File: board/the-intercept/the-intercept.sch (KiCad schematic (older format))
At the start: 35 parts, among them J1 USB_B_Micro, Q1 Q_Photo_NPN, SW1 SW_Push, SW2 SW_Push, U1 ESP32-WROOM-32D, U2 93LCxxB, U3 FT232H, U4 LM1117-3.3, Y1 12MHz

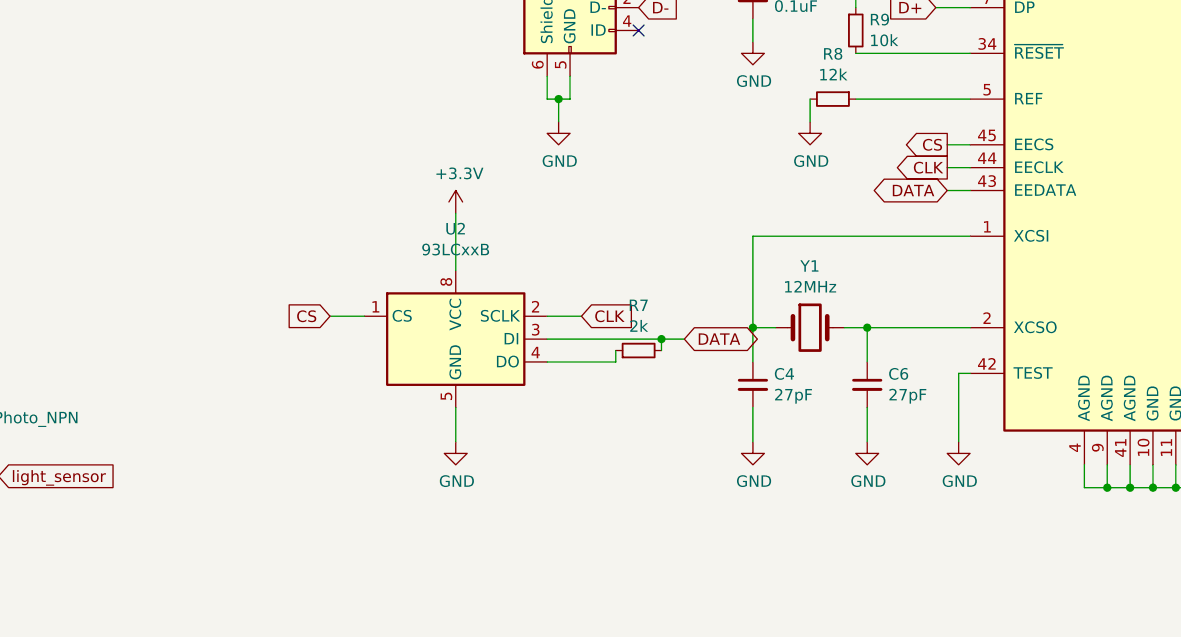
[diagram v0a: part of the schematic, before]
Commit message: Revision two of the board
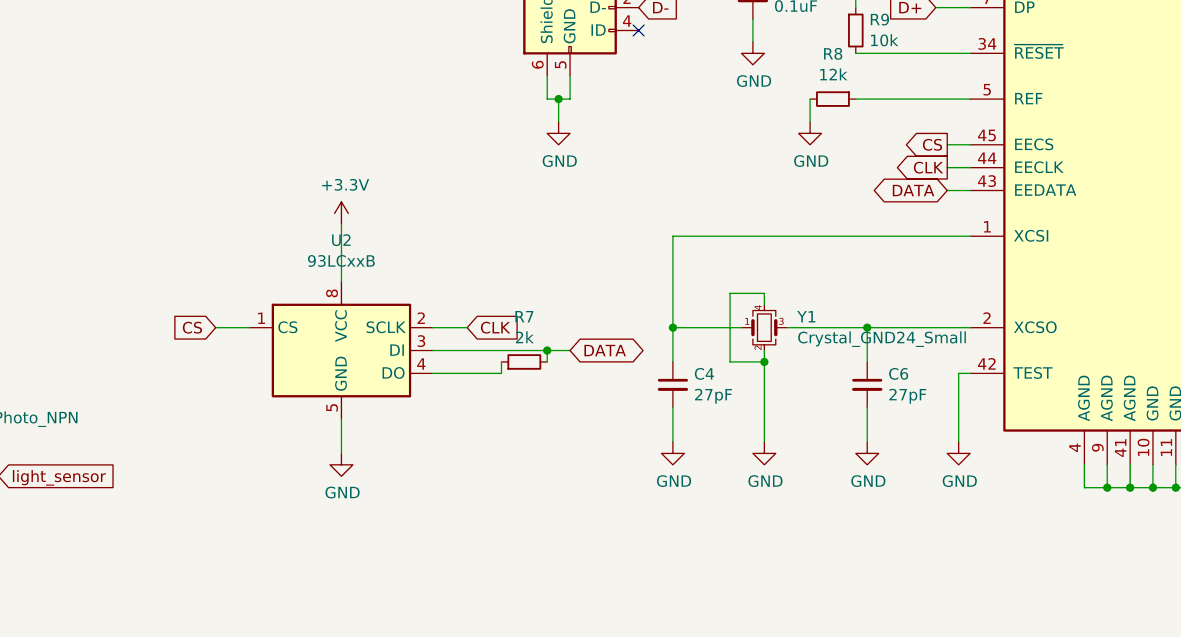
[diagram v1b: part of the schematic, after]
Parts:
- removed Y1: 12MHz, Crystal:Crystal_SMD_Abracon_ABM8G-4Pin_3.2x2.5mm, symbol Device:Crystal
- added Y1: Crystal_GND24_Small, Crystal:Crystal_SMD_Abracon_ABM8G-4Pin_3.2x2.5mm, symbol Device:Crystal_GND24_Small
- U2: footprint Package_SO:SOIC-8-1EP_3.9x4.9mm_P1.27mm_EP2.29x3mm -> Package_SO:SOIC-8_3.9x4.9mm_P1.27mm
- U3: footprint Package_QFP:LQFP-48-1EP_7x7mm_P0.5mm_EP3.6x3.6mm -> Package_QFP:LQFP-48_7x7mm_P0.5mm
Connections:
- net GND: now also Y1.2, Y1.4
- net at C4.1, U3.1 (XCSI): now also Y1.1
- net at C6.1, U3.2 (XCSO): now also Y1.3
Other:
- moved on the sheet: C4, R7, U2
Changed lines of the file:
@@
 F 0 "U3" H 9050 5931 50  0000 C CNN
 F 1 "FT232H" H 9050 5840 50  0000 C CNN
-F 2 "Package_QFP:LQFP-48-1EP_7x7mm_P0.5mm_EP3.6x3.6mm" H 9050 4250 50  0001 C CNN
+F 2 "Package_QFP:LQFP-48_7x7mm_P0.5mm" H 9050 4250 50  0001 C CNN
 F 3 "http://www.ftdichip.com/Products/ICs/FT232H.htm" H 9050 4250 50  0001 C CNN
 	1    9050 4250
@@
 Wire Wire Line
 	9150 5850 9150 6000
-$Comp
-L Device:Crystal Y1
-U 1 1 5CBBFE5E
-P 7450 5150
-F 0 "Y1" H 7450 5418 50  0000 C CNN
-F 1 "12MHz" H 7450 5327 50  0000 C CNN
-F 2 "Crystal:Crystal_SMD_Abracon_ABM8G-4Pin_3.2x2.5mm" H 7450 5150 50  0001 C CNN
-F 3 "~" H 7450 5150 50  0001 C CNN
-	1    7450 5150
-	1    0    0    -1
-$EndComp
-$Comp
-L Device:C_Small C4
-U 1 1 5CBC360A
-P 7200 5400
-F 0 "C4" H 7292 5446 50  0000 L CNN
-F 1 "27pF" H 7292 5355 50  0000 L CNN
-F 2 "Capacitor_SMD:C_0603_1608Metric" H 7200 5400 50  0001 C CNN
-F 3 "~" H 7200 5400 50  0001 C CNN
-	1    7200 5400
-	1    0    0    -1
-$EndComp
-Wire Wire Line
-	7200 5150 7300 5150
-Wire Wire Line
-	7200 4750 7200 5150
-Wire Wire Line
-	8150 4750 7200 4750
-Wire Wire Line
-	7200 5150 7200 5300
-Connection ~ 7200 5150
+Wire Wire Line
+	6850 4750 6850 5150
+Wire Wire Line
+	6850 5150 6850 5300
+Connection ~ 6850 5150
 $Comp
 L power:GND #PWR0103
 U 1 1 5CBC6BBE
-P 7200 5650
-F 0 "#PWR0103" H 7200 5400 50  0001 C CNN
-F 1 "GND" H 7205 5477 50  0000 C CNN
-F 2 "" H 7200 5650 50  0001 C CNN
-F 3 "" H 7200 5650 50  0001 C CNN
-	1    7200 5650
+P 6850 5650
+F 0 "#PWR0103" H 6850 5400 50  0001 C CNN
+F 1 "GND" H 6855 5477 50  0000 C CNN
+F 2 "" H 6850 5650 50  0001 C CNN
+F 3 "" H 6850 5650 50  0001 C CNN
+	1    6850 5650
 	1    0    0    -1
 $EndComp
@@
 	7700 5500 7700 5650
 Wire Wire Line
-	7200 5500 7200 5650
+	6850 5500 6850 5650
 Wire Wire Line
 	7700 5300 7700 5150
-Connection ~ 7700 5150
-Wire Wire Line
-	7700 5150 7600 5150
 Wire Wire Line
 	7700 5150 8150 5150
@@
 L power:GND #PWR07
 U 1 1 5CDF624D
-P 5900 5650
-F 0 "#PWR07" H 5900 5400 50  0001 C CNN
-F 1 "GND" H 5905 5477 50  0000 C CNN
-F 2 "" H 5900 5650 50  0001 C CNN
-F 3 "" H 5900 5650 50  0001 C CNN
-	1    5900 5650
-	1    0    0    -1
-$EndComp
-Wire Wire Line
-	5900 5500 5900 5650
+P 5400 5700
+F 0 "#PWR07" H 5400 5450 50  0001 C CNN
+F 1 "GND" H 5405 5527 50  0000 C CNN
+F 2 "" H 5400 5700 50  0001 C CNN
+F 3 "" H 5400 5700 50  0001 C CNN
+	1    5400 5700
+	1    0    0    -1
+$EndComp
+Wire Wire Line
+	5400 5550 5400 5700
 $Comp
 L power:+3.3V #PWR06
 U 1 1 5CDFF462
-P 5900 4650
-F 0 "#PWR06" H 5900 4500 50  0001 C CNN
-F 1 "+3.3V" H 5915 4823 50  0000 C CNN
-F 2 "" H 5900 4650 50  0001 C CNN
-F 3 "" H 5900 4650 50  0001 C CNN
-	1    5900 4650
-	1    0    0    -1
-$EndComp
-Wire Wire Line
-	5900 4650 5900 4900
+P 5400 4700
+F 0 "#PWR06" H 5400 4550 50  0001 C CNN
+F 1 "+3.3V" H 5415 4873 50  0000 C CNN
+F 2 "" H 5400 4700 50  0001 C CNN
+F 3 "" H 5400 4700 50  0001 C CNN
+	1    5400 4700
+	1    0    0    -1
+$EndComp
+Wire Wire Line
+	5400 4700 5400 4950
 Wire Wire Line
 	8150 4450 8050 4450
@@
 Text GLabel 8050 4550 0    50   BiDi ~ 0
 DATA
-Text GLabel 5350 5100 0    50   Input ~ 0
-CS
-Text GLabel 6450 5100 2    50   Input ~ 0
+Text GLabel 5950 5150 2    50   Input ~ 0
 CLK
 $Comp
 L Device:R_Small R7
 U 1 1 5CE2C99B
-P 6700 5250
-F 0 "R7" V 6896 5250 50  0000 C CNN
-F 1 "2k" V 6805 5250 50  0000 C CNN
-F 2 "Resistor_SMD:R_0603_1608Metric" H 6700 5250 50  0001 C CNN
-F 3 "~" H 6700 5250 50  0001 C CNN
-	1    6700 5250
+P 6200 5300
+F 0 "R7" V 6396 5300 50  0000 C CNN
+F 1 "2k" V 6305 5300 50  0000 C CNN
+F 2 "Resistor_SMD:R_0603_1608Metric" H 6200 5300 50  0001 C CNN
+F 3 "~" H 6200 5300 50  0001 C CNN
+	1    6200 5300
 	0    -1   -1   0
 $EndComp
 Wire Wire Line
-	6800 5200 6800 5250
-Wire Wire Line
-	6300 5200 6800 5200
-Wire Wire Line
-	6800 5200 6900 5200
-Connection ~ 6800 5200
-Wire Wire Line
-	6600 5300 6600 5250
-Wire Wire Line
-	6300 5300 6600 5300
-Text GLabel 6900 5200 2    50   BiDi ~ 0
+	6300 5250 6300 5300
+Wire Wire Line
+	5800 5250 6300 5250
+Wire Wire Line
+	6300 5250 6400 5250
+Connection ~ 6300 5250
+Wire Wire Line
+	6100 5350 6100 5300
+Wire Wire Line
+	5800 5350 6100 5350
+Text GLabel 6400 5250 2    50   BiDi ~ 0
 DATA
 $Comp
@@
 	8150 4350 8050 4350
 Wire Wire Line
-	6300 5100 6450 5100
-Wire Wire Line
-	5500 5100 5350 5100
+	5800 5150 5950 5150
+Wire Wire Line
+	5000 5150 4850 5150
 Text GLabel 8050 4450 0    50   Output ~ 0
 CLK
@@
 L Memory_EEPROM:93LCxxB U2
 U 1 1 5D1A17AE
-P 5900 5200
-F 0 "U2" H 5900 5681 50  0000 C CNN
-F 1 "93LCxxB" H 5900 5590 50  0000 C CNN
-F 2 "Package_SO:SOIC-8-1EP_3.9x4.9mm_P1.27mm_EP2.29x3mm" H 5900 5200 50  0001 C CNN
-F 3 "http://ww1.microchip.com/downloads/en/DeviceDoc/20001749K.pdf" H 5900 5200 50  0001 C CNN
-	1    5900 5200
+P 5400 5250
+F 0 "U2" H 5400 5731 50  0000 C CNN
+F 1 "93LCxxB" H 5400 5640 50  0000 C CNN
+F 2 "Package_SO:SOIC-8_3.9x4.9mm_P1.27mm" H 5400 5250 50  0001 C CNN
+F 3 "http://ww1.microchip.com/downloads/en/DeviceDoc/20001749K.pdf" H 5400 5250 50  0001 C CNN
+	1    5400 5250
 	1    0    0    -1
 $EndComp
@@
 	1    0    0    -1
 $EndComp
+$Comp
+L Device:Crystal_GND24_Small Y1
+U 1 1 5CC9CC3C
+P 7250 5150
+F 0 "Y1" H 7394 5196 50  0000 L CNN
+F 1 "Crystal_GND24_Small" H 7394 5105 50  0000 L CNN
+F 2 "Crystal:Crystal_SMD_Abracon_ABM8G-4Pin_3.2x2.5mm" H 7250 5150 50  0001 C CNN
+F 3 "~" H 7250 5150 50  0001 C CNN
+	1    7250 5150
+	1    0    0    -1
+$EndComp
+$Comp
+L power:GND #PWR017
+U 1 1 5CCF4162
+P 7250 5650
+F 0 "#PWR017" H 7250 5400 50  0001 C CNN
+F 1 "GND" H 7255 5477 50  0000 C CNN
+F 2 "" H 7250 5650 50  0001 C CNN
+F 3 "" H 7250 5650 50  0001 C CNN
+	1    7250 5650
+	1    0    0    -1
+$EndComp
+Wire Wire Line
+	7250 5250 7250 5300
+Wire Wire Line
+	7250 5050 7250 5000
+Wire Wire Line
+	7250 5000 7100 5000
+Wire Wire Line
+	7100 5000 7100 5300
+Wire Wire Line
+	7100 5300 7250 5300
+Connection ~ 7250 5300
+Wire Wire Line
+	7250 5300 7250 5650
+$Comp
+L Device:C_Small C4
+U 1 1 5CBC360A
+P 6850 5400
+F 0 "C4" H 6942 5446 50  0000 L CNN
+F 1 "27pF" H 6942 5355 50  0000 L CNN
+F 2 "Capacitor_SMD:C_0603_1608Metric" H 6850 5400 50  0001 C CNN
+F 3 "~" H 6850 5400 50  0001 C CNN
+	1    6850 5400
+	1    0    0    -1
+$EndComp
+Wire Wire Line
+	6850 5150 7150 5150
+Wire Wire Line
+	7350 5150 7700 5150
+Connection ~ 7700 5150
+Wire Wire Line
+	6850 4750 8150 4750
+Text GLabel 4850 5150 0    50   Input ~ 0
+CS
 $EndSCHEMATC
